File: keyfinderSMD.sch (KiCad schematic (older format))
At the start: 23 parts, among them Q1 2N7002, U1 4049

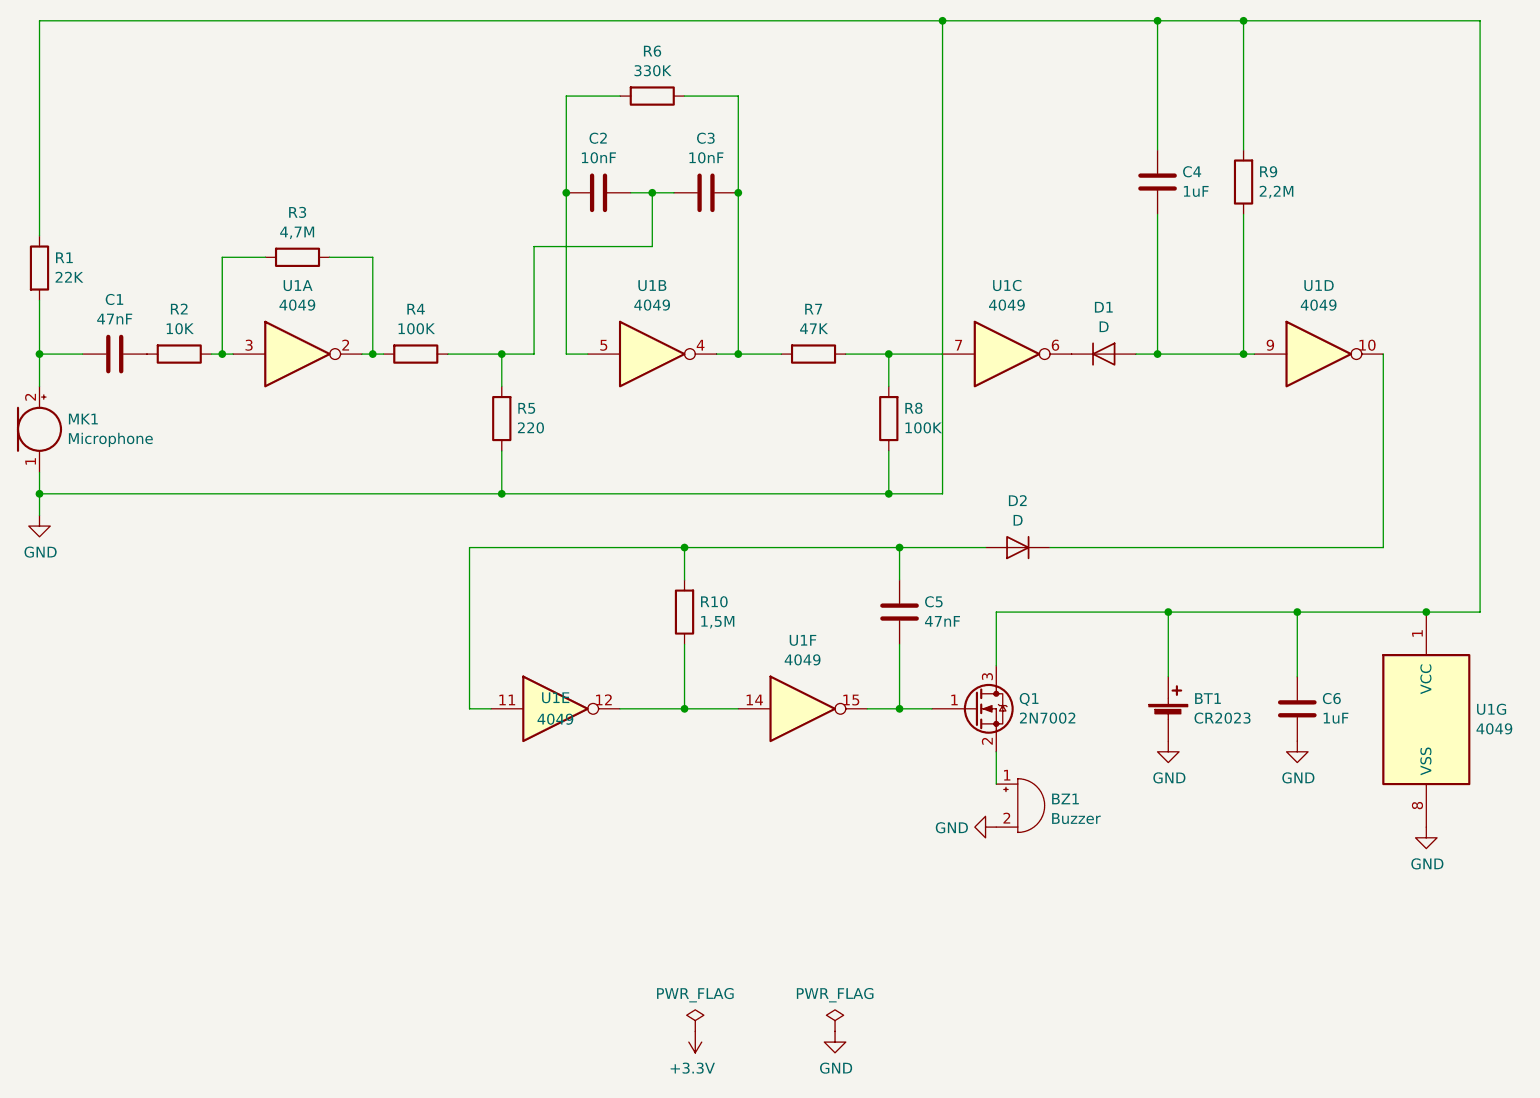
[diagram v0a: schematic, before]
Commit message: added first draft
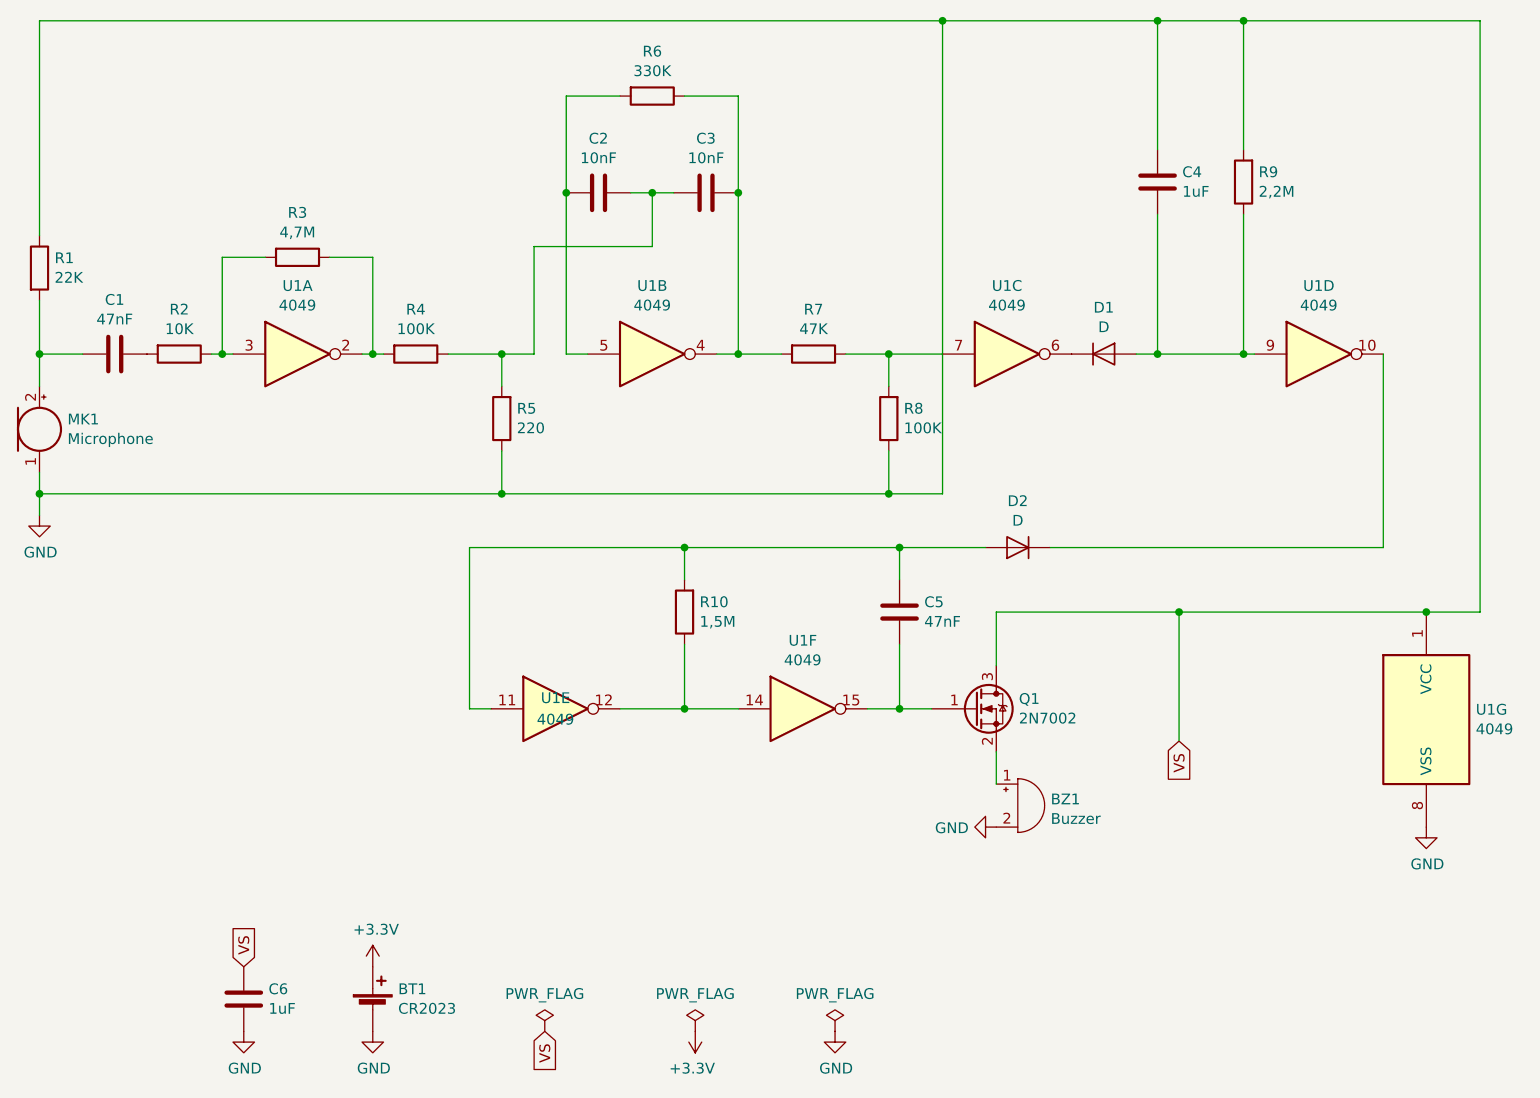
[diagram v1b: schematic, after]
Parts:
- BZ1: footprint Buzzer_Beeper:Buzzer_12x9.5RM7.6 -> keyfinderSMD:Buzzer_12x9.5RM7.6
- MK1: footprint (none) -> keyfinderSMD:MicrophoneDIP
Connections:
- net +3V3: now also BT1.1 (+)
- net GND: no longer BT1.1 (+)
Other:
- moved on the sheet: BT1, C6
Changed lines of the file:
@@
 L Device:Battery_Cell BT1
 U 1 1 5C052186
-P 7800 5300
-F 0 "BT1" H 7918 5396 50  0000 L CNN
-F 1 "CR2023" H 7918 5305 50  0000 L CNN
-F 2 "Battery:BatteryHolder_Keystone_1060_1x2032" V 7800 5360 50  0001 C CNN
-F 3 "~" V 7800 5360 50  0001 C CNN
-	1    7800 5300
+P 4100 6650
+F 0 "BT1" H 4218 6746 50  0000 L CNN
+F 1 "CR2023" H 4218 6655 50  0000 L CNN
+F 2 "Battery:BatteryHolder_Keystone_1060_1x2032" V 4100 6710 50  0001 C CNN
+F 3 "~" V 4100 6710 50  0001 C CNN
+	1    4100 6650
 	1    0    0    -1
 $EndComp
@@
 L power:GND #PWR0102
 U 1 1 5C0521C4
-P 7800 5400
-F 0 "#PWR0102" H 7800 5150 50  0001 C CNN
-F 1 "GND" H 7805 5227 50  0000 C CNN
-F 2 "" H 7800 5400 50  0001 C CNN
-F 3 "" H 7800 5400 50  0001 C CNN
-	1    7800 5400
+P 4100 6750
+F 0 "#PWR0102" H 4100 6500 50  0001 C CNN
+F 1 "GND" H 4105 6577 50  0000 C CNN
+F 2 "" H 4100 6750 50  0001 C CNN
+F 3 "" H 4100 6750 50  0001 C CNN
+	1    4100 6750
 	1    0    0    -1
 $EndComp
@@
 L Device:C C6
 U 1 1 5C052287
-P 8400 5250
-F 0 "C6" H 8515 5296 50  0000 L CNN
-F 1 "1uF" H 8515 5205 50  0000 L CNN
-F 2 "Capacitor_SMD:C_0805_2012Metric_Pad1.15x1.40mm_HandSolder" H 8438 5100 50  0001 C CNN
-F 3 "~" H 8400 5250 50  0001 C CNN
-	1    8400 5250
+P 3500 6600
+F 0 "C6" H 3615 6646 50  0000 L CNN
+F 1 "1uF" H 3615 6555 50  0000 L CNN
+F 2 "Capacitor_SMD:C_0805_2012Metric_Pad1.15x1.40mm_HandSolder" H 3538 6450 50  0001 C CNN
+F 3 "~" H 3500 6600 50  0001 C CNN
+	1    3500 6600
 	1    0    0    -1
 $EndComp
@@
 L power:GND #PWR0104
 U 1 1 5C0522CD
-P 8400 5400
-F 0 "#PWR0104" H 8400 5150 50  0001 C CNN
-F 1 "GND" H 8405 5227 50  0000 C CNN
-F 2 "" H 8400 5400 50  0001 C CNN
-F 3 "" H 8400 5400 50  0001 C CNN
-	1    8400 5400
+P 3500 6750
+F 0 "#PWR0104" H 3500 6500 50  0001 C CNN
+F 1 "GND" H 3505 6577 50  0000 C CNN
+F 2 "" H 3500 6750 50  0001 C CNN
+F 3 "" H 3500 6750 50  0001 C CNN
+	1    3500 6750
 	1    0    0    -1
 $EndComp
@@
 F 0 "MK1" H 2680 3996 50  0000 L CNN
 F 1 "Microphone" H 2680 3905 50  0000 L CNN
-F 2 "" V 2550 4050 50  0001 C CNN
+F 2 "keyfinderSMD:MicrophoneDIP" V 2550 4050 50  0001 C CNN
 F 3 "~" V 2550 4050 50  0001 C CNN
 	1    2550 3950
@@
 F 0 "BZ1" H 7253 5729 50  0000 L CNN
 F 1 "Buzzer" H 7253 5638 50  0000 L CNN
-F 2 "Buzzer_Beeper:Buzzer_12x9.5RM7.6" V 7075 5800 50  0001 C CNN
+F 2 "keyfinderSMD:Buzzer_12x9.5RM7.6" V 7075 5800 50  0001 C CNN
 F 3 "~" V 7075 5800 50  0001 C CNN
 	1    7100 5700
@@
 Wire Wire Line
 	7000 5600 7000 5450
-Wire Wire Line
-	7800 5100 7800 4800
-Connection ~ 7800 4800
-Wire Wire Line
-	7800 4800 7000 4800
-Wire Wire Line
-	8400 5100 8400 4800
-Connection ~ 8400 4800
-Wire Wire Line
-	8400 4800 7800 4800
 $Comp
 L 4xxx:4049 U1
@@
 $EndComp
 Connection ~ 9000 4800
-Wire Wire Line
-	9000 4800 8400 4800
 $Comp
 L power:GND #PWR0107
@@
 	1    0    0    -1
 $EndComp
+$Comp
+L power:PWR_FLAG #FLG0103
+U 1 1 5C081956
+P 4900 6750
+F 0 "#FLG0103" H 4900 6825 50  0001 C CNN
+F 1 "PWR_FLAG" H 4900 6924 50  0000 C CNN
+F 2 "" H 4900 6750 50  0001 C CNN
+F 3 "~" H 4900 6750 50  0001 C CNN
+	1    4900 6750
+	1    0    0    -1
+$EndComp
+Text GLabel 4900 6750 3    50   Input ~ 0
+VS
+Wire Wire Line
+	7000 4800 7850 4800
+Text GLabel 7850 5400 3    50   Input ~ 0
+VS
+Wire Wire Line
+	7850 5400 7850 4800
+Connection ~ 7850 4800
+$Comp
+L power:+3.3V #PWR0108
+U 1 1 5C08486B
+P 4100 6450
+F 0 "#PWR0108" H 4100 6300 50  0001 C CNN
+F 1 "+3.3V" H 4115 6623 50  0000 C CNN
+F 2 "" H 4100 6450 50  0001 C CNN
+F 3 "" H 4100 6450 50  0001 C CNN
+	1    4100 6450
+	1    0    0    -1
+$EndComp
+Wire Wire Line
+	7850 4800 9000 4800
+Text GLabel 3500 6450 1    50   Input ~ 0
+VS
 $EndSCHEMATC
